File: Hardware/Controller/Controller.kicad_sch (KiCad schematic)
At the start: 18 parts, among them J1 MPU6050_Connector, J2 Conn_01x02_Socket, SW1 SW_Push, SW2 SW_Push, SW3 SW_Push, SW4 SW_Push, SW5 100SP1T1B1M2QEH, SW6 100SP1T1B1M2QEH, SW7 Slide Switch, U1 AMS1117-3.3, U2 DM-OLED096-636, U3 LM2596S-5

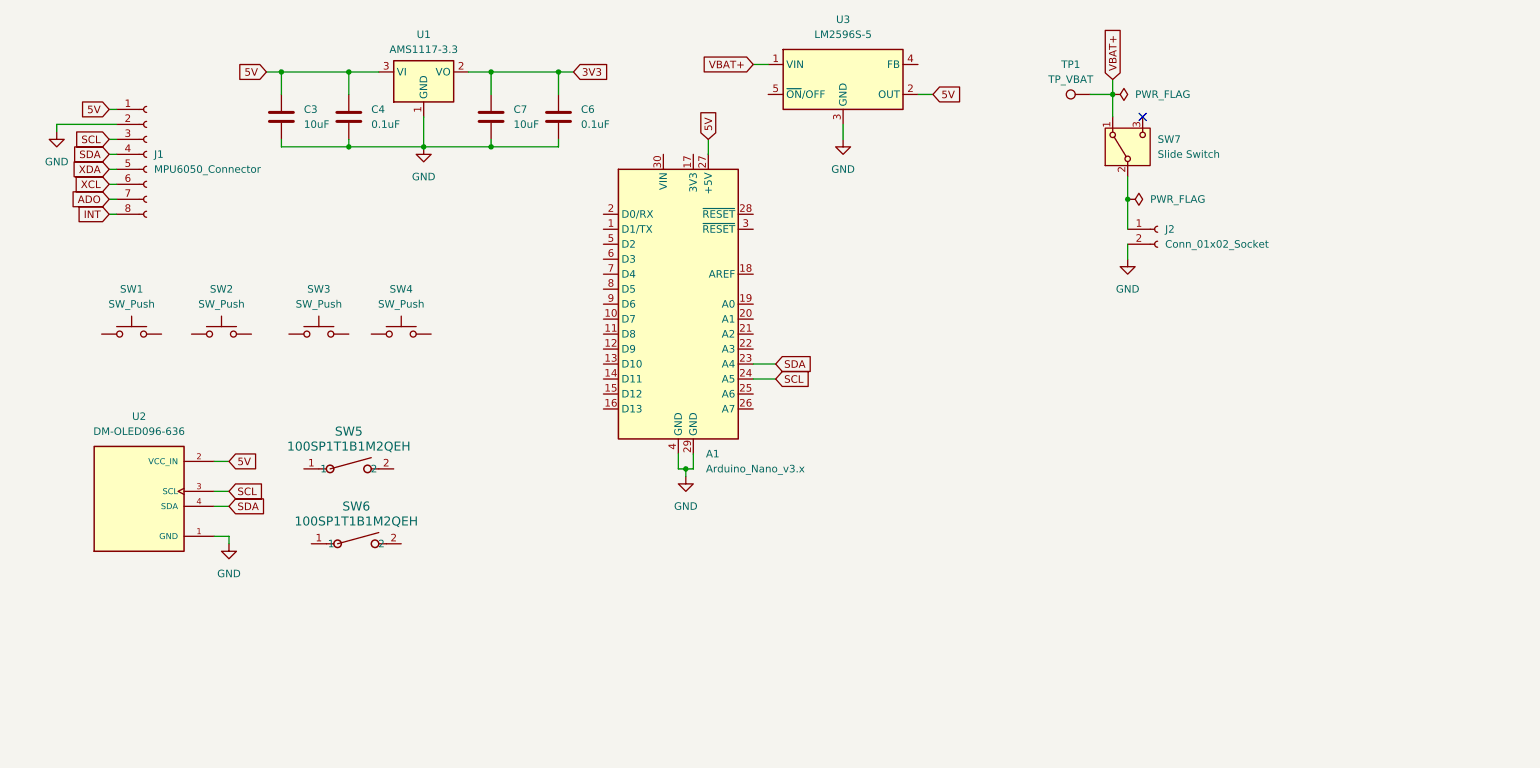
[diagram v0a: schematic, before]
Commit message: PCB Schematic initiated
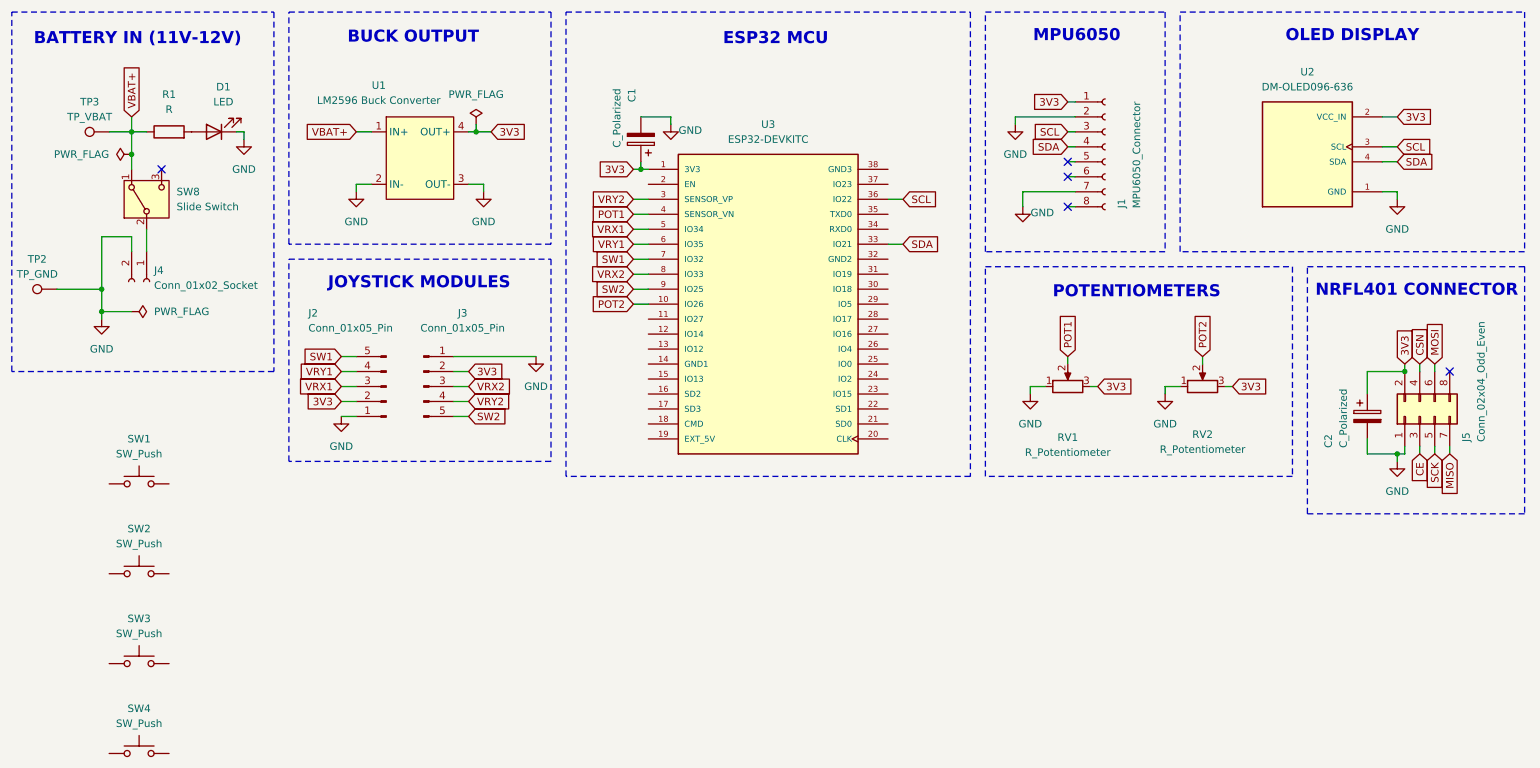
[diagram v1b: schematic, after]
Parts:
- removed A1: Arduino_Nano_v3.x, Module:Arduino_Nano, symbol MCU_Module:Arduino_Nano_v3.x
- removed C3, C7: 10uF, Capacitor_SMD:C_0805_2012Metric, symbol Device:C
- removed C4, C6: 0.1uF, Capacitor_SMD:C_0603_1608Metric, symbol Device:C
- removed J2: Conn_01x02_Socket, symbol Connector:Conn_01x02_Socket
- removed SW5, SW6: 100SP1T1B1M2QEH, SW_100SP1T_12P7X6P86_EWI, symbol 3P Toggle Switch:100SP1T1B1M2QEH
- removed SW7: Slide Switch, Button_Switch_THT:SW_Slide-03_Wuerth-WS-SLTV_10x2.5x6.4_P2.54mm, symbol Switch:SW_SPDT
- removed TP1: TP_VBAT, TestPoint:TestPoint_Pad_2.0x2.0mm, symbol Connector:TestPoint
- removed U1: AMS1117-3.3, Package_TO_SOT_SMD:SOT-223-3_TabPin2, symbol Regulator_Linear:AMS1117-3.3
- removed U3: LM2596S-5, Package_TO_SOT_SMD:TO-263-5_TabPin3, symbol Regulator_Switching:LM2596S-5
- added C1, C2: C_Polarized, symbol Device:C_Polarized
- added D1: LED, symbol Device:LED
- added J2, J3: Conn_01x05_Pin, symbol Connector:Conn_01x05_Pin
- added J4: Conn_01x02_Socket, symbol Connector:Conn_01x02_Socket
- added J5: Conn_02x04_Odd_Even, symbol Connector_Generic:Conn_02x04_Odd_Even
- added R1: R, symbol Device:R
- added RV1, RV2: R_Potentiometer, symbol Device:R_Potentiometer
- added SW8: Slide Switch, Button_Switch_THT:SW_Slide-03_Wuerth-WS-SLTV_10x2.5x6.4_P2.54mm, symbol Switch:SW_SPDT
- added TP2: TP_GND, TestPoint:TestPoint_Pad_2.0x2.0mm, symbol Connector:TestPoint
- added TP3: TP_VBAT, TestPoint:TestPoint_Pad_2.0x2.0mm, symbol Connector:TestPoint
- added U1: LM2596 Buck Converter, Buck_Converter:LM2596_Buck_Module, symbol buck_converter:LM2596_Module
- added U3: ESP32-DEVKITC, ESP32-DEVKITC:MODULE_ESP32-DEVKITC, symbol ESP32-DEVKITC:ESP32-DEVKITC
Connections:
- net 5V is gone; now on net 3V3: J1.1 (Pin_1), U2.2 (VCC_IN)
- net ADO is gone; now on net GND: J1.7 (Pin_7)
- net 3V3: now also C1.1, C2.1, J2.2 (Pin_2), J3.2 (Pin_2), J5.2 (Pin_2), RV1.3, RV2.3, U1.4 (OUT+), U3.1 (3V3)
- net GND: now also C1.2, C2.2, D1.1 (K), J2.1 (Pin_1), J3.1 (Pin_1), J4.2 (Pin_2), J5.1 (Pin_1), RV1.1, RV2.1, TP2.1, U1.2 (IN-), U1.3 (OUT-)
- net SCL: now also U3.36 (IO22)
- net SDA: now also U3.33 (IO21)
- net VBAT+: now also R1.1, SW8.1 (A), TP3.1, U1.1 (IN+)
- net INT: no longer names the net of J1.8 (Pin_8)
- net XCL: no longer names the net of J1.6 (Pin_6)
- net XDA: no longer names the net of J1.5 (Pin_5)
- new net: D1.2 (A), R1.2
- new net: J4.1 (Pin_1), SW8.2 (B)
- new net CE: J5.3 (Pin_3)
- new net CSN: J5.4 (Pin_4)
- new net MISO: J5.7 (Pin_7)
- new net MOSI: J5.6 (Pin_6)
- new net POT1: RV1.2, U3.4 (SENSOR_VN)
- new net POT2: RV2.2, U3.10 (IO26)
- new net SCK: J5.5 (Pin_5)
- new net SW1: J2.5 (Pin_5), U3.7 (IO32)
- new net SW2: J3.5 (Pin_5), U3.9 (IO25)
- new net VRX1: J2.3 (Pin_3), U3.5 (IO34)
- new net VRX2: J3.3 (Pin_3), U3.8 (IO33)
- new net VRY1: J2.4 (Pin_4), U3.6 (IO35)
- new net VRY2: J3.4 (Pin_4), U3.3 (SENSOR_VP)
- no-connect marks 1 -> 5
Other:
- note added: "BATTERY IN (11V-12V)"
- note added: "BUCK OUTPUT"
- note added: "ESP32 MCU"
- note added: "JOYSTICK MODULES"
- note added: "MPU6050"
- note added: "NRFL401 CONNECTOR"
- note added: "OLED DISPLAY"
- note added: "POTENTIOMETERS"
- moved on the sheet: J1, SW1, SW2, SW3, SW4, U2

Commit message: PCB Schematic started
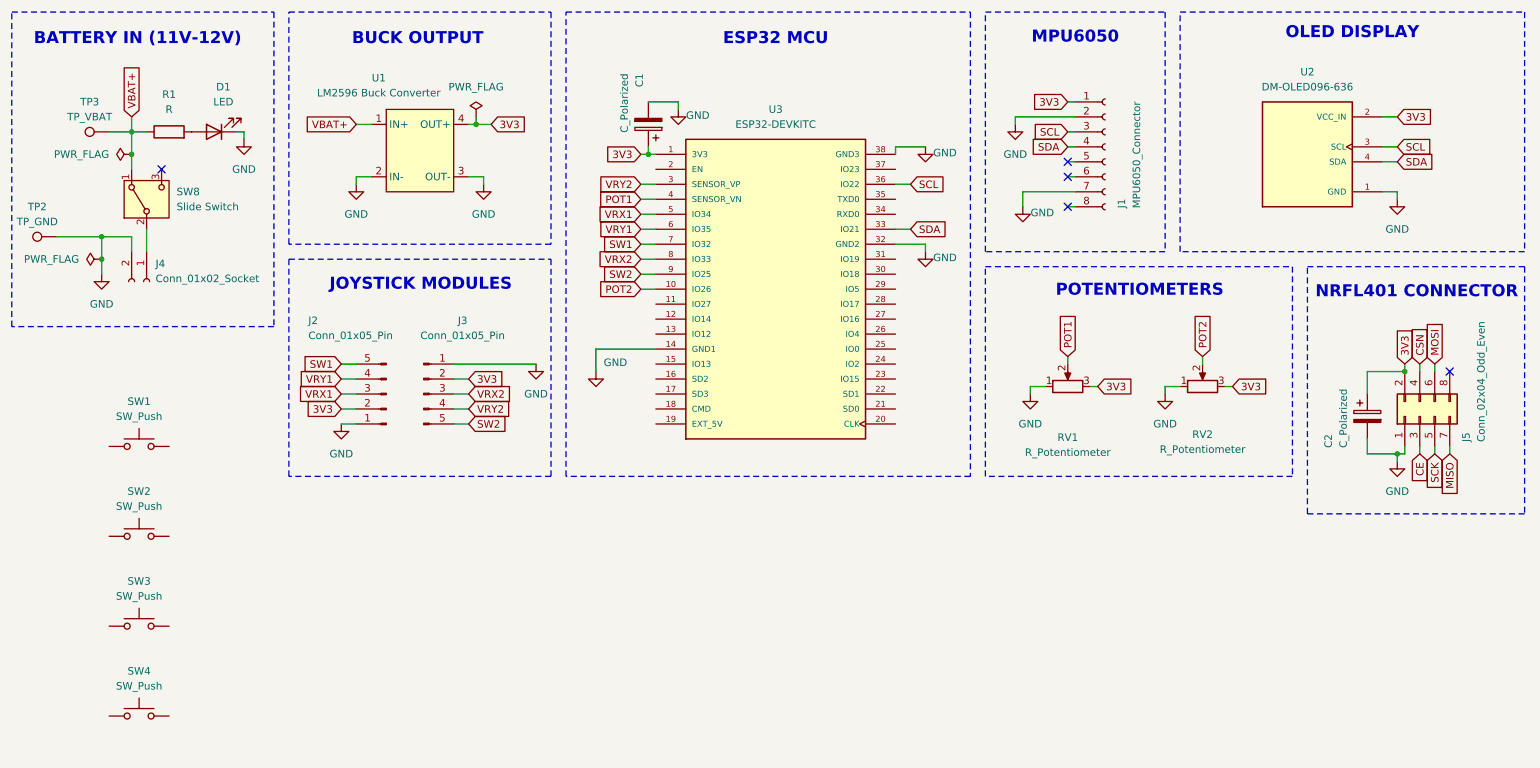
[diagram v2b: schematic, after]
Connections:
- net GND: now also U3.14 (GND1), U3.32 (GND2), U3.38 (GND3)
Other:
- moved on the sheet: C1, J2, J3, SW1, SW2, SW3, SW4, TP2, U1, U3
